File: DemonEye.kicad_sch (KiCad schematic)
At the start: 51 parts, among them CN1 PicoBlade 1x06 P1.25mm, Q1 CSD25501F3, Q2 CSD25501F3, Q3 BC807-25QAZ, Q4 CSD25501F3, Q5 BC807-25QAZ, Q6 CSD25501F3, Q7 BC807-25QAZ, Q8 CSD25501F3, Q9 BC807-25QAZ, U1 WS2814F, U2 TLV76701DRVx

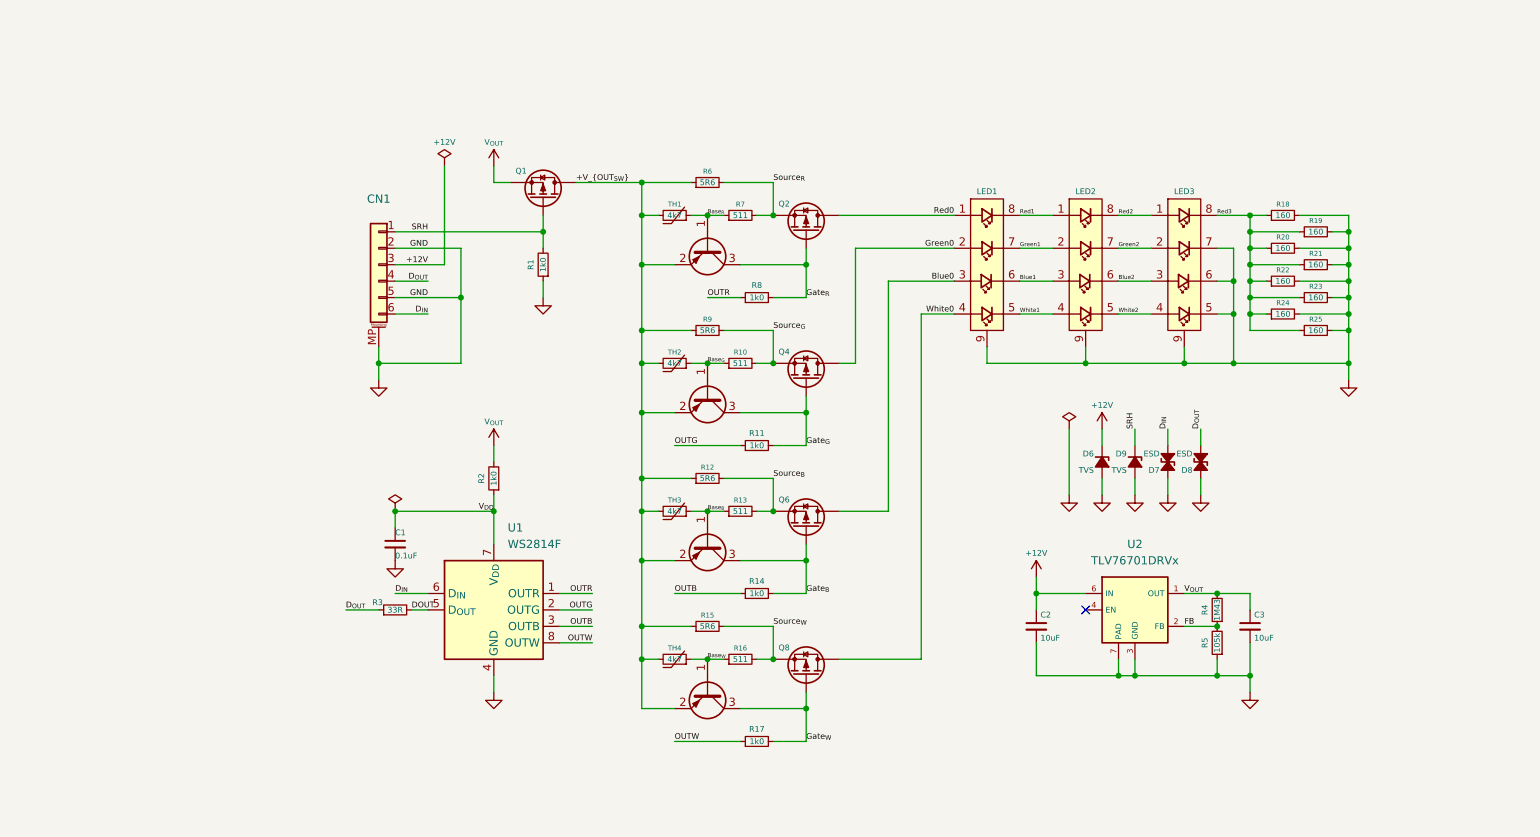
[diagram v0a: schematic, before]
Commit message: Update DemonEye.kicad_pcb, DemonEye.kicad_prl, DemonEye.kicad_pro, and 8 more files
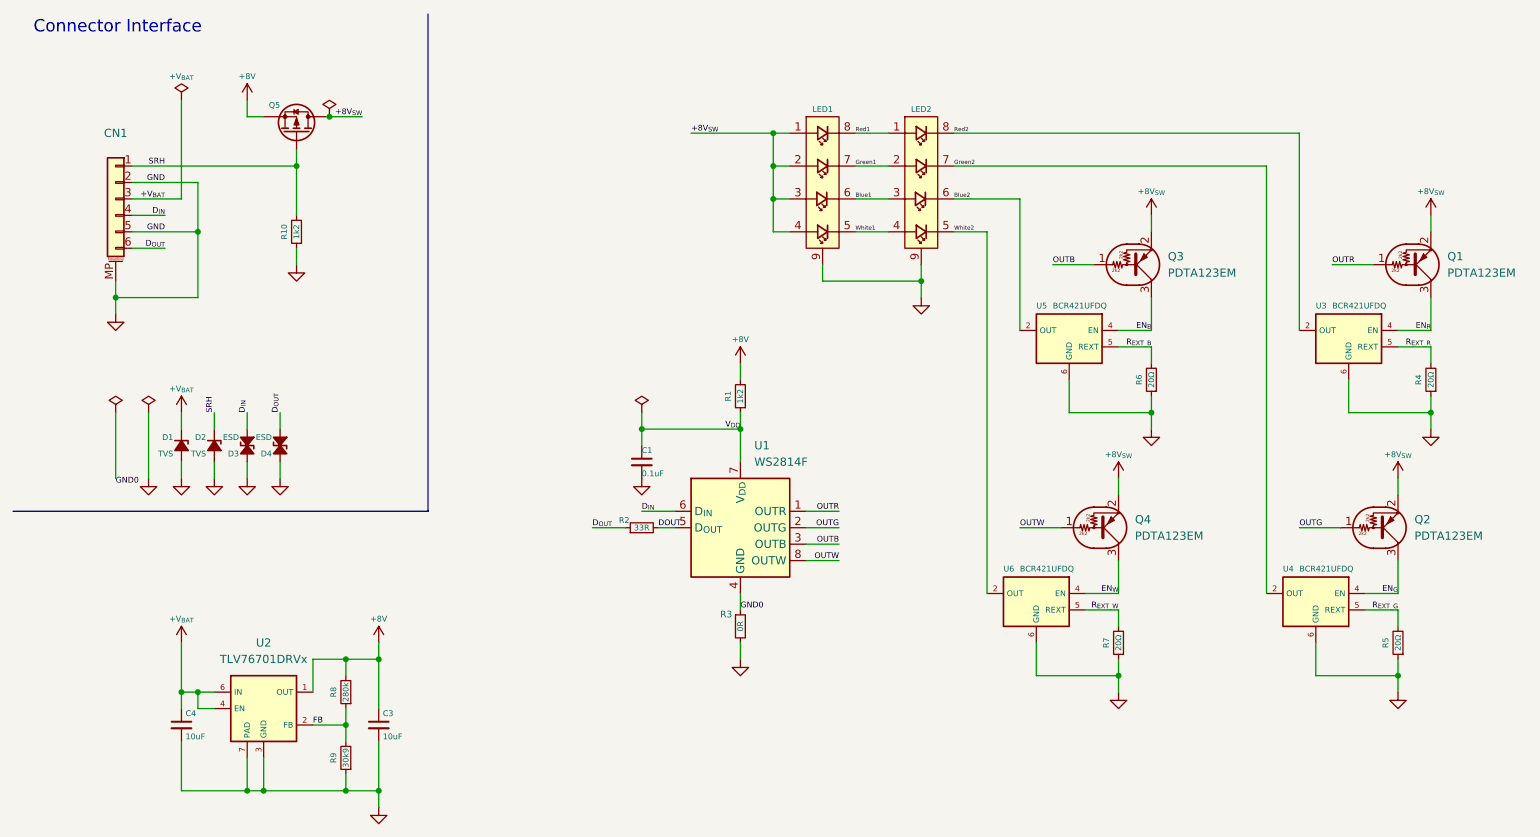
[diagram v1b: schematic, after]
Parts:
- removed LED3: QLSP06RGBXWAJ, Personal_FootprintLibrary:QLSP06RGBXWAJ, symbol PersonalSchematicSymbolLibrary:QLSP06RGBXWAJ
- removed Q2, Q4, Q6, Q8: CSD25501F3, My Package_Leadless:Texas_-YJN_0.7x0.6mm_PicoStar, symbol PersonalSchematicSymbolLibrary:Q_PMOS
- removed Q3, Q5, Q7, Q9: BC807-25QAZ, My Package_Leadless:DFN1010D-3, symbol PersonalSchematicSymbolLibrary:Q_PNP_BEC
- removed R10, R13, R16: 511, My Resistors:R_0201_Dense, symbol Device:R_Small
- removed R11, R14, R17, R8: 1k0, My Resistors:R_0402_Nominal, symbol Device:R_Small
- removed R12, R15, R9: 5R6, My Resistors:R_0402_Nominal, symbol Device:R_Small
- removed R18, R19, R20, R21, R22, R23, R24, R25: 160, My Resistors:R_0201_Dense, symbol Device:R_Small
- removed TH1, TH2, TH3, TH4: 4k7, My Resistors:TH_0402_Nominal, symbol PersonalSchematicSymbolLibrary:TH_Small
- added Q1, Q2, Q3, Q4: PDTA123EM, My Package_Leadless:Diodes_DFN1006-3, symbol PersonalSchematicSymbolLibrary:DTA123E
- added R3: 0R, My Resistors:R_0402_Nominal, symbol Device:R_Small
- added R4, R5: 20Ω, My Resistors:R_0201_Dense, symbol Device:R_Small
- added U3, U4, U5, U6: BCR421UFDQ, DemonEye_Footprints:BCR421UFDQ, symbol My Power Management:BCR421UFDQ
- R1: renamed from R2; value 1k0 -> 1k2; footprint My Resistors:R_0402_Nominal -> My Resistors:R_0201_Dense; Distributor Link 1 https://www.digikey.com/en/products/detail/yageo/AC0402FR-7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 -> https://www.digikey.com/en/products/detail/yageo/AC0201FR-0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; Distributor Link 2 https://www.mouser.com/ProductDetail/YAGEO/AC0402FR-7W1KL?q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 -> https://www.mouser.com/ProductDetail/YAGEO/AC0201FR-071K2L?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; LCSC C5455561 -> C226448; Manufacturer Part Number AC0402FR-7W1KL -> AC0201FR-071K2L
- R10: renamed from R1; value 1k0 -> 1k2; footprint My Resistors:R_0402_Nominal -> My Resistors:R_0201_Dense; Distributor Link 1 https://www.digikey.com/en/products/detail/yageo/AC0402FR-7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 -> https://www.digikey.com/en/products/detail/yageo/AC0201FR-0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; Distributor Link 2 https://www.mouser.com/ProductDetail/YAGEO/AC0402FR-7W1KL?q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 -> https://www.mouser.com/ProductDetail/YAGEO/AC0201FR-071K2L?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; LCSC C5455561 -> C226448; Manufacturer Part Number AC0402FR-7W1KL -> AC0201FR-071K2L
- R2: renamed from R3; footprint My Resistors:R_0201_Nominal -> My Resistors:R_0201_Dense
- R6: value 5R6 -> 20Ω; footprint My Resistors:R_0402_Nominal -> My Resistors:R_0201_Dense; Distributor Link 1 https://www.digikey.com/en/products/detail/koa-speer-electr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 -> https://www.digikey.com/en/products/detail/yageo/AC0201FR-0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; Distributor Link 2 https://www.mouser.com/ProductDetail/KOA-Speer/RK73H1ETTP5R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 -> https://www.mouser.com/ProductDetail/YAGEO/AC0201FR-0720RL?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; LCSC C830259 -> C226464; Manufacturer KOA Speer Elec -> YAGEO; Manufacturer Part Number RK73H1ETTP5R60F -> AC0201FR-0720RL
- R7: value 511 -> 20Ω; Distributor Link 1 https://www.digikey.com/en/products/detail/walsin-technolog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 -> https://www.digikey.com/en/products/detail/yageo/AC0201FR-0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; Distributor Link 2 https://www.mouser.com/ProductDetail/Walsin/WR02X5110FAL?qs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 -> https://www.mouser.com/ProductDetail/YAGEO/AC0201FR-0720RL?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; LCSC C367646 -> C226464; Manufacturer Walsin Tech Corp -> YAGEO; Manufacturer Part Number WR02X5110FAL -> AC0201FR-0720RL
- R8: renamed from R4; value 1M43 -> 280k; Distributor Link 2 https://www.mouser.com/ProductDetail/Royalohm/0201WMF1434TE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 -> https://www.mouser.com/ProductDetail/Royalohm/0201WMF2803TE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; LCSC C784121 -> C778392; Manufacturer Part Number (none) -> 0201WMF2803TEE
- R9: renamed from R5; value 105k -> 30k9; Distributor Link 1 https://www.digikey.com/en/products/detail/yageo/AC0201FR-0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 -> (none); Distributor Link 2 https://www.mouser.com/ProductDetail/YAGEO/AC0201FR-07105KL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 -> https://www.mouser.com/ProductDetail/Royalohm/0201WMF3092TE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; LCSC C226397 -> C473585; Manufacturer YAGEO -> UNI-ROYAL(Uniroyal Elec); Manufacturer Part Number AC0201FR-07105KL -> 0201WMF3092TEE
- renumbered C2 to C4, D6 to D1, D9 to D2, D7 to D3, D8 to D4, Q1 to Q5
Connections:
- net +12V is gone; now on net +V_{BAT}: C4.1, CN1.3 (Pin_3), D1.1 (K), U2.6 (IN)
- net Base_{R} is gone; now on net GND: R7.1
- net Blue0 is gone; now on net +8V_{SW}: LED1.3 (Blue_A)
- net Green0 is gone; now on net +8V_{SW}: LED1.2 (Green_A)
- net Red0 is gone; now on net +8V_{SW}: LED1.1 (Red_A)
- net White0 is gone; now on net +8V_{SW}: LED1.4 (White_A)
- net Blue2: now also U5.2 (OUT)
- net D_{IN}: now also CN1.4 (Pin_4); no longer CN1.6 (Pin_4)
- net D_{OUT}: now also CN1.6 (Pin_4); no longer CN1.4 (Pin_4)
- net GND: now also R6.1, R3.2, R4.1, R5.1, U3.6 (GND), U4.6 (GND), U5.6 (GND), U6.6 (GND); no longer U1.4 (GND)
- net Green2: now also U4.2 (OUT)
- net OUTB: now also Q3.1 (B)
- net OUTG: now also Q2.1 (B)
- net OUTR: now also Q1.1 (B)
- net OUTW: now also Q4.1 (B)
- net Red2: now also U3.2 (OUT)
- net White2: now also U6.2 (OUT)
- net +V_{BAT}: now reaches U2.4 (EN)
- net +V_{OUT_{SW}} renamed +8V_{SW}
- net +8V_{SW}: now also Q1.2 (E), Q2.2 (E), Q3.2 (E), Q4.2 (E); no longer R6.1
- net Source_{R} renamed R_{EXT_B}
- net R_{EXT_B}: now also U5.5 (REXT); no longer R7.2
- net V_{OUT} renamed +8V
- new net EN_{B}: Q3.3 (C), U5.4 (EN)
- new net EN_{G}: Q2.3 (C), U4.4 (EN)
- new net EN_{R}: Q1.3 (C), U3.4 (EN)
- new net EN_{W}: Q4.3 (C), U6.4 (EN)
- new net GND0: R3.1, U1.4 (GND)
- new net R_{EXT_G}: R5.2, U4.5 (REXT)
- new net R_{EXT_R}: R4.2, U3.5 (REXT)
- new net R_{EXT_W}: R7.2, U6.5 (REXT)
- no-connect marks 1 -> 0
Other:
- note added: "Connector Interface"
- moved on the sheet: C1, C3, C4, CN1, D1, D2, D3, D4, LED1, LED2, Q5, R1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
